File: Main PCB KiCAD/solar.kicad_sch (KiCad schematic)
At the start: 28 parts, among them J7 Solar in, SW1 SW_SPDT, U1 TPS54331D

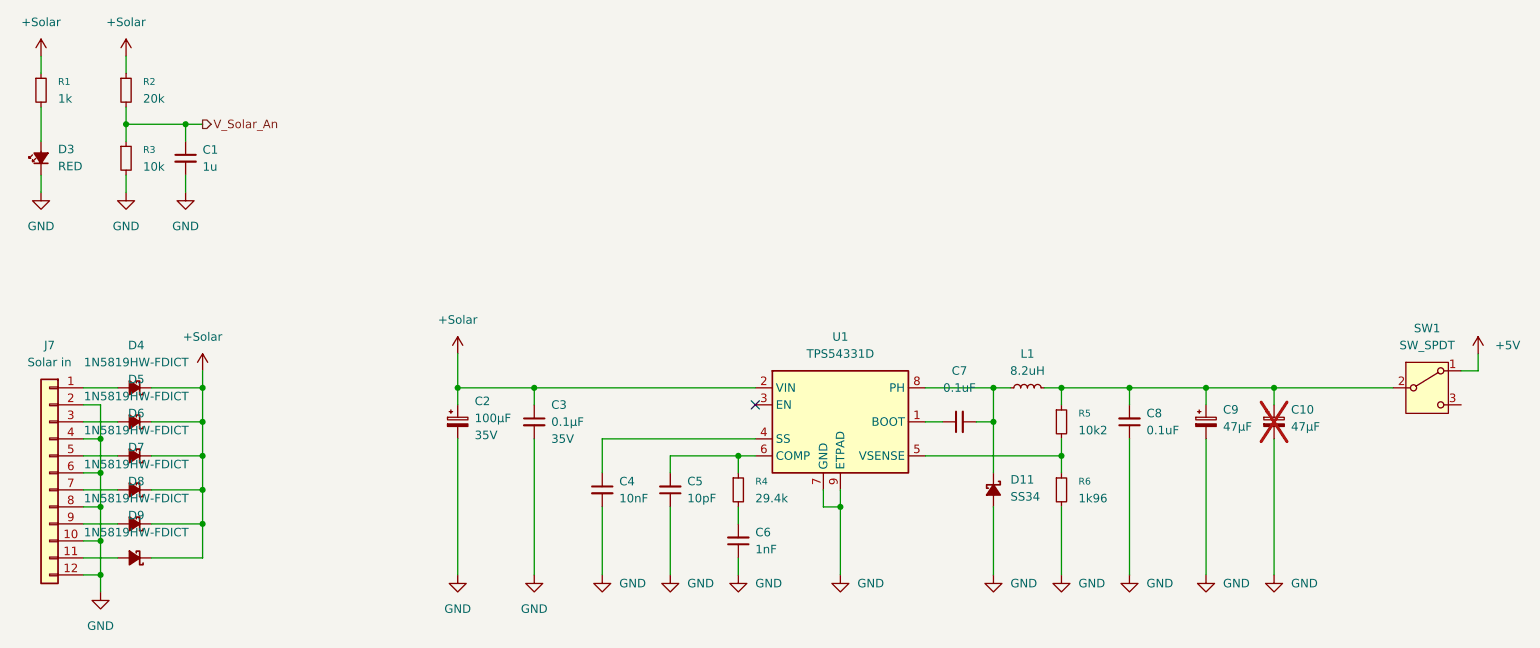
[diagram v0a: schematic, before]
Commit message: .
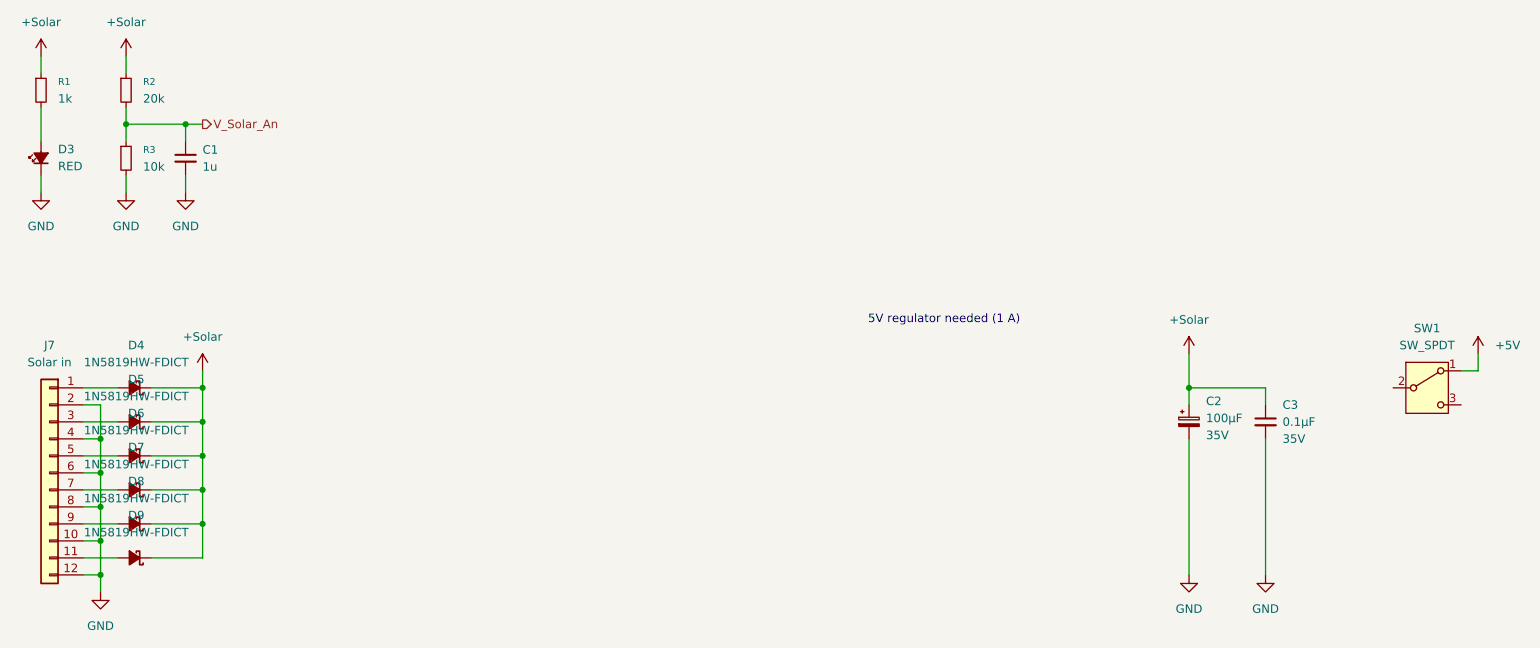
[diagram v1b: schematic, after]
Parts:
- removed C10, C9: 47μF, Capacitor_SMD:CP_Elec_5x5.9, symbol Device:C_Polarized_Small
- removed C4: 10nF, Capacitor_SMD:C_0805_2012Metric_Pad1.18x1.45mm_HandSolder, symbol Device:C_Small
- removed C5: 10pF, Capacitor_SMD:C_0805_2012Metric_Pad1.18x1.45mm_HandSolder, symbol Device:C_Small
- removed C6: 1nF, Capacitor_SMD:C_0805_2012Metric_Pad1.18x1.45mm_HandSolder, symbol Device:C_Small
- removed C7, C8: 0.1uF, Capacitor_SMD:C_0805_2012Metric_Pad1.18x1.45mm_HandSolder, symbol Device:C_Small
- removed D11: SS34, Diode_SMD:D_SMA_Handsoldering, symbol Device:D_Schottky_Small_Filled
- removed L1: 8.2uH, Inductor_SMD:L_Taiyo-Yuden_NR-60xx_HandSoldering, symbol Device:L_Small
- removed R4: 29.4k, Resistor_SMD:R_0805_2012Metric_Pad1.20x1.40mm_HandSolder, symbol Device:R_Small
- removed R5: 10k2, Resistor_SMD:R_0805_2012Metric_Pad1.20x1.40mm_HandSolder, symbol Device:R_Small
- removed R6: 1k96, Resistor_SMD:R_0805_2012Metric_Pad1.20x1.40mm_HandSolder, symbol Device:R_Small
- removed U1: TPS54331D, Package_SO:TI_SO-PowerPAD-8_ThermalVias, symbol Regulator_Switching:TPS54336ADDA
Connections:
- no-connect marks 1 -> 0
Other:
- note added: "5V regulator needed (1 A)"
- moved on the sheet: C2, C3
